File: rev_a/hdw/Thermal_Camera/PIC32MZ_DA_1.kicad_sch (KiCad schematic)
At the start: 3 parts

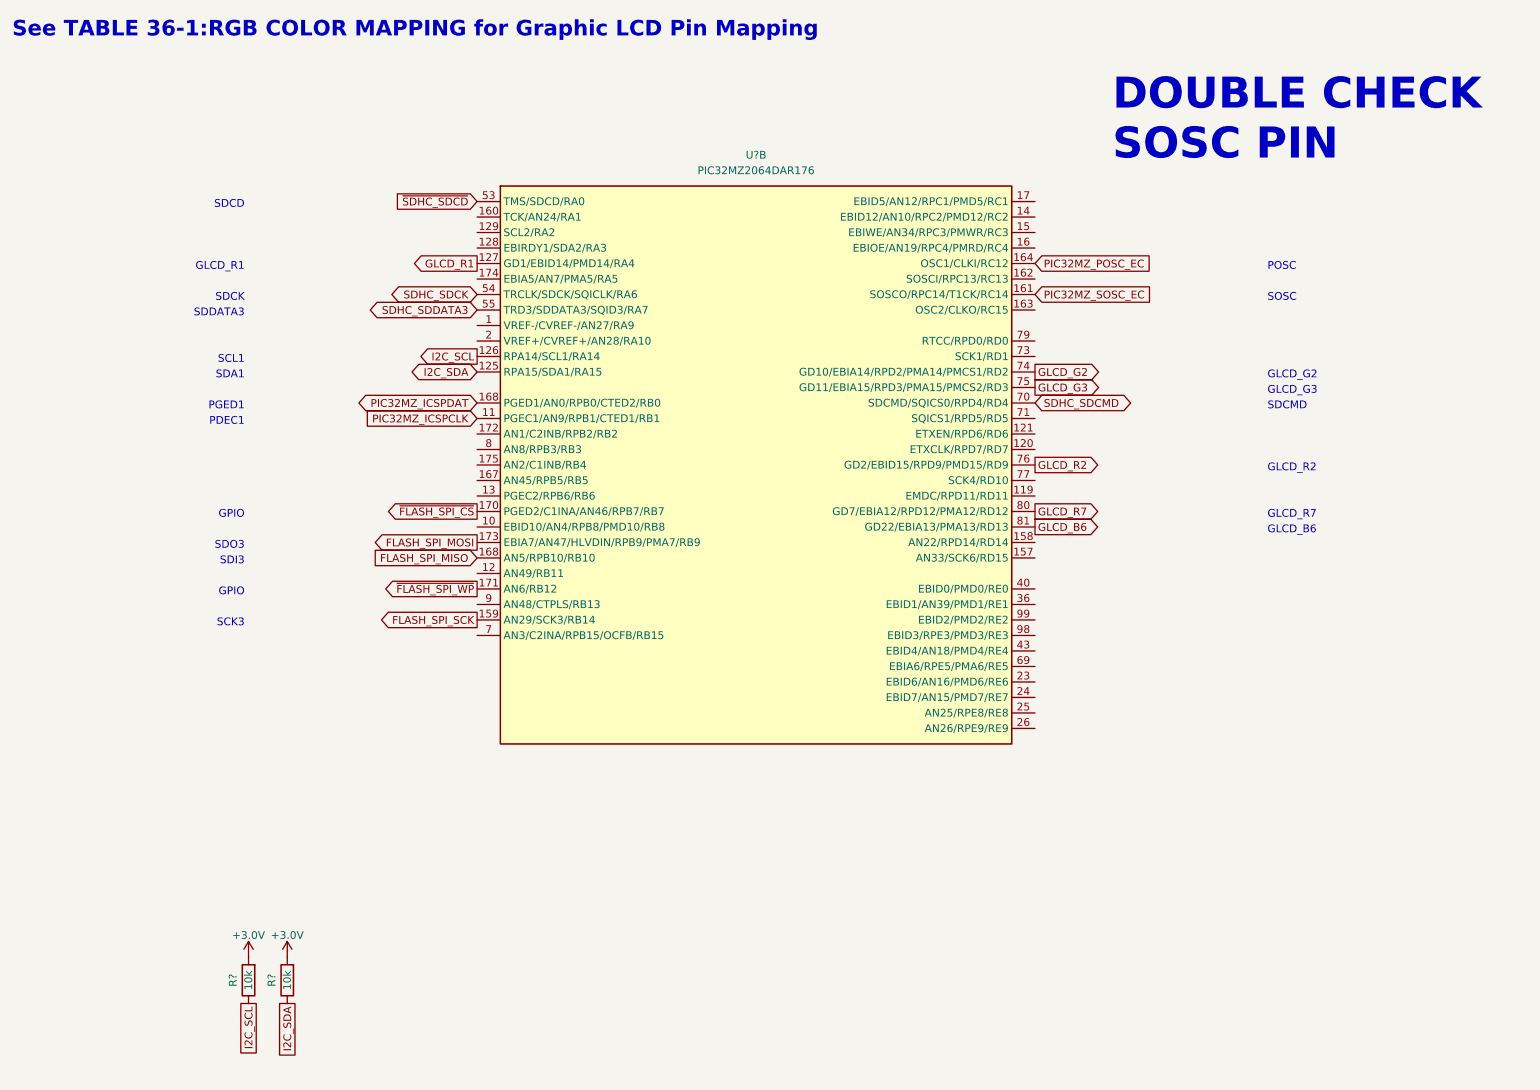
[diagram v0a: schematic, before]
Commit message: blah blah
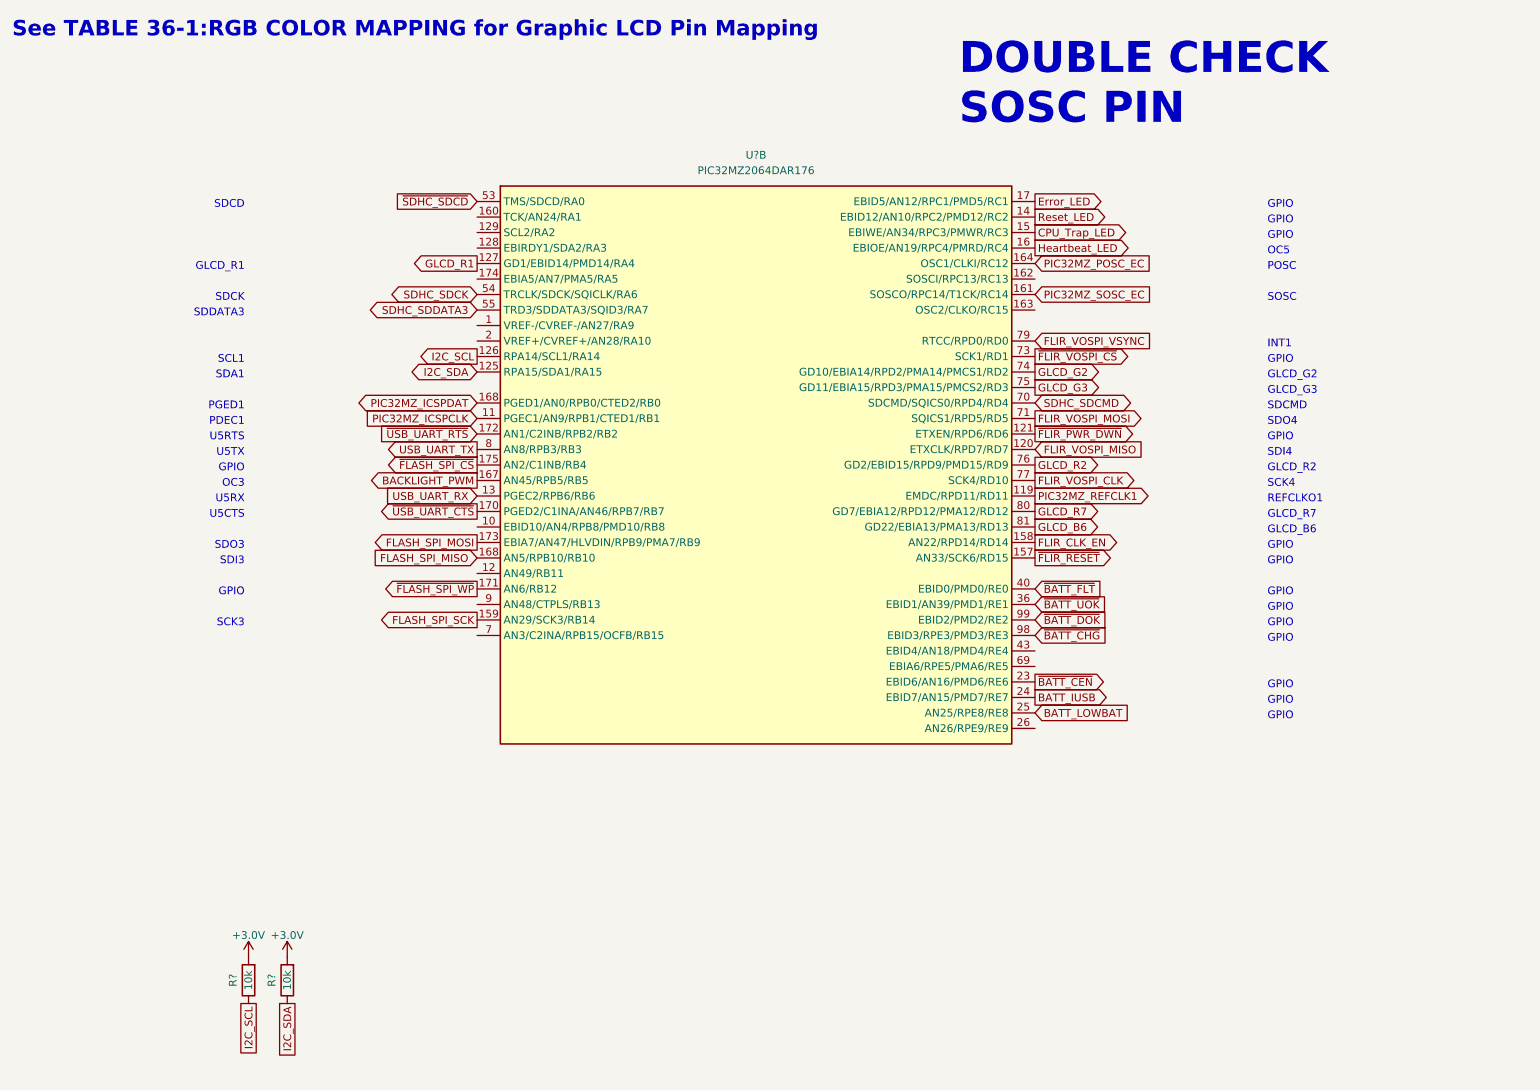
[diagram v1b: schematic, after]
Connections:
- net ~{FLASH_SPI_CS}: now also U?.175 (AN2/C1INB/RB4); no longer U?.170 (PGED2/C1INA/AN46/RPB7/RB7)
- net PIC32MZ_REFCLK1: now reaches U?.119 (EMDC/RPD11/RD11)
- net FLIR_VOSPI_MISO: now reaches U?.120 (ETXCLK/RPD7/RD7)
- net ~{FLIR_PWR_DWN}: now reaches U?.121 (ETXEN/RPD6/RD6)
- net USB_UART_RX: now reaches U?.13 (PGEC2/RPB6/RB6)
- net Reset_LED: now reaches U?.14 (EBID12/AN10/RPC2/PMD12/RC2)
- net CPU_Trap_LED: now reaches U?.15 (EBIWE/AN34/RPC3/PMWR/RC3)
- net ~{FLIR_RESET}: now reaches U?.157 (AN33/SCK6/RD15)
- net FLIR_CLK_EN: now reaches U?.158 (AN22/RPD14/RD14)
- net Heartbeat_LED: now reaches U?.16 (EBIOE/AN19/RPC4/PMRD/RC4)
- net BACKLIGHT_PWM: now reaches U?.167 (AN45/RPB5/RB5)
- net Error_LED: now reaches U?.17 (EBID5/AN12/RPC1/PMD5/RC1)
- net ~{USB_UART_RTS}: now reaches U?.172 (AN1/C2INB/RPB2/RB2)
- net ~{BATT_CEN}: now reaches U?.23 (EBID6/AN16/PMD6/RE6)
- net BATT_IUSB: now reaches U?.24 (EBID7/AN15/PMD7/RE7)
- net BATT_LOWBAT: now reaches U?.25 (AN25/RPE8/RE8)
- net ~{BATT_UOK}: now reaches U?.36 (EBID1/AN39/PMD1/RE1)
- net ~{BATT_FLT}: now reaches U?.40 (EBID0/PMD0/RE0)
- net FLIR_VOSPI_MOSI: now reaches U?.71 (SQICS1/RPD5/RD5)
- net ~{FLIR_VOSPI_CS}: now reaches U?.73 (SCK1/RD1)
- net FLIR_VOSPI_CLK: now reaches U?.77 (SCK4/RD10)
- net FLIR_VOSPI_VSYNC: now reaches U?.79 (RTCC/RPD0/RD0)
- net USB_UART_TX: now reaches U?.8 (AN8/RPB3/RB3)
- net ~{BATT_CHG}: now reaches U?.98 (EBID3/RPE3/PMD3/RE3)
- net ~{BATT_DOK}: now reaches U?.99 (EBID2/PMD2/RE2)
- new net ~{USB_UART_CTS}: U?.170 (PGED2/C1INA/AN46/RPB7/RB7)
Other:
- note added: "INT1"
- note added: "OC3"
- note added: "OC5"
- note added: "REFCLKO1"
- note added: "SCK4"
- note added: "SDI4"
- note added: "SDO4"
- note added: "U5CTS"
- note added: "U5RTS"
- note added: "U5RX"
- note added: "U5TX"
